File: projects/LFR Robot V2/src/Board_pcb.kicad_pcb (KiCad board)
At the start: 2 copper layers, 77.5 x 103 mm, 0 parts

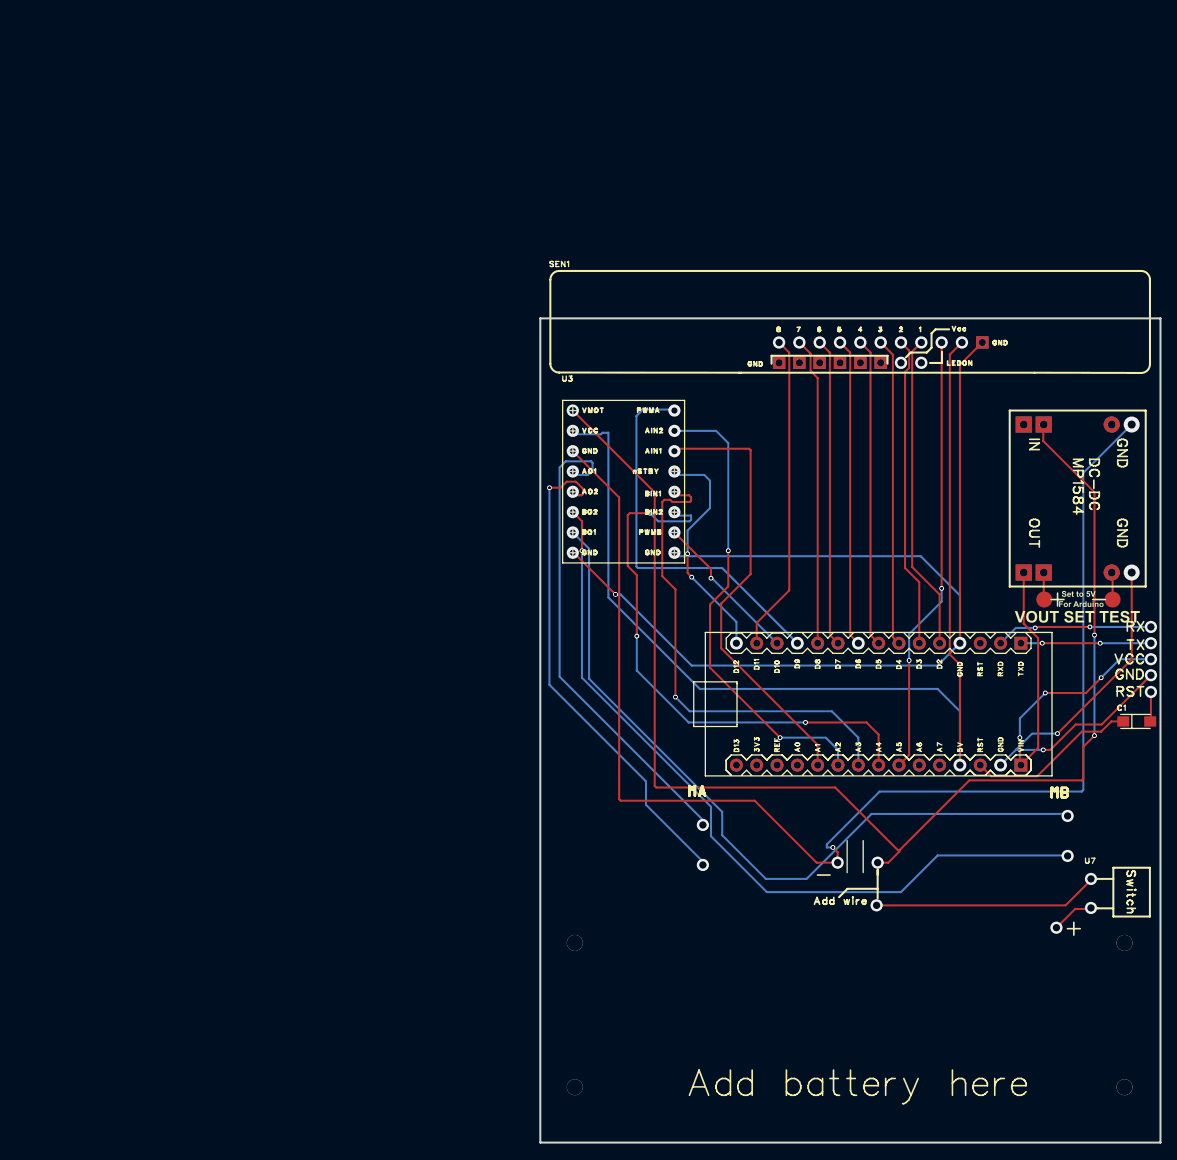
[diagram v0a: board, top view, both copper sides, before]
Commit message: Add files via upload
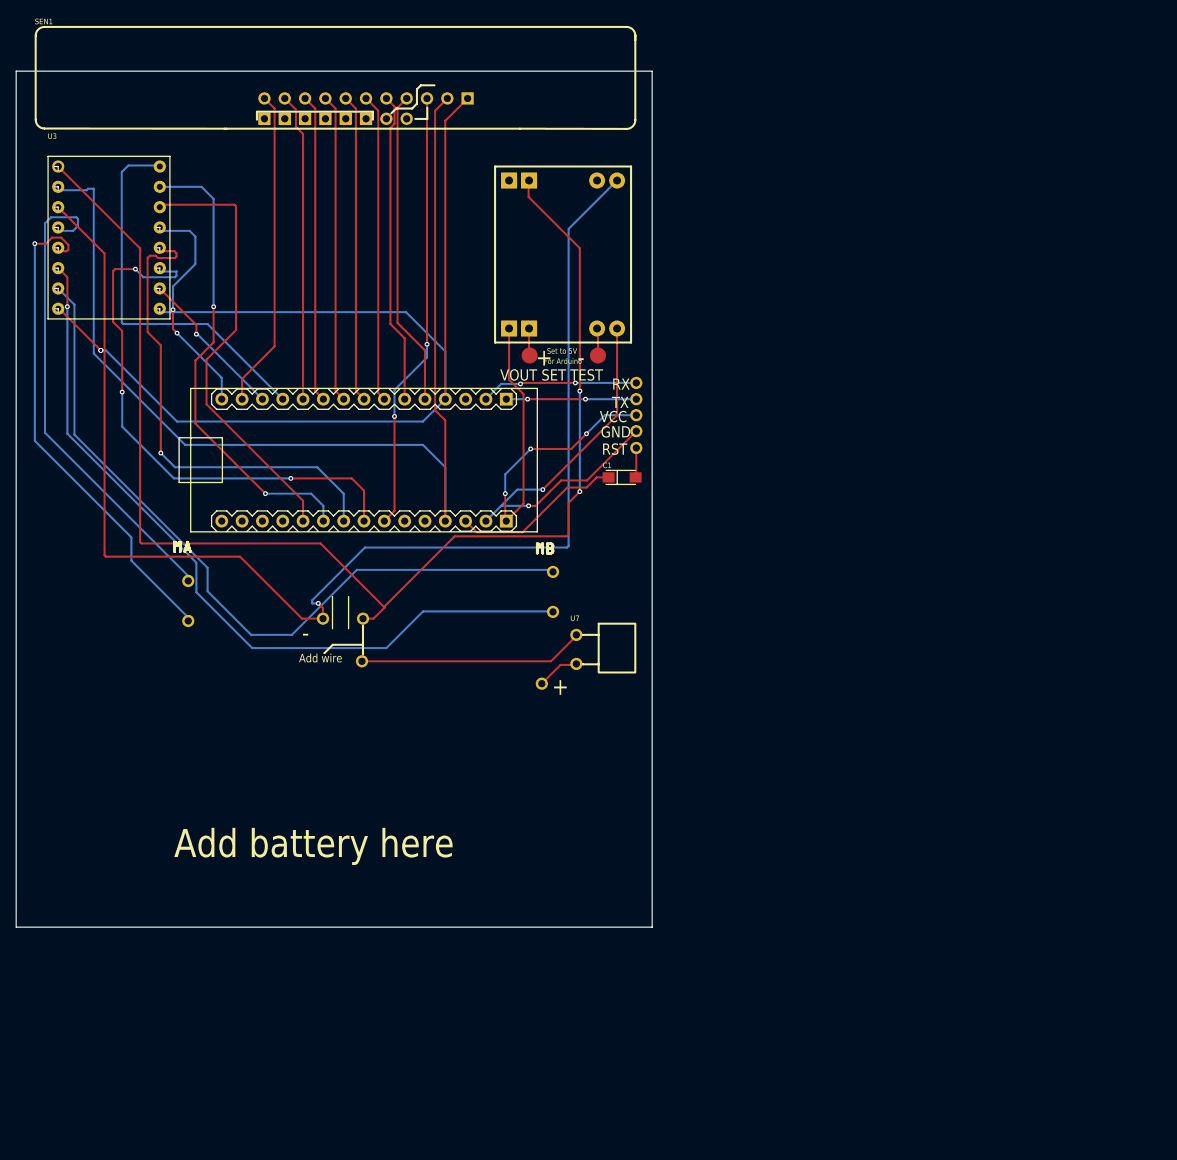
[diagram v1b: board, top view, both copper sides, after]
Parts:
- added ?: , LFR V2:Pad_e140, F.Cu at (195.5, 79.1)
- added ?: , LFR V2:Pad_e431, F.Cu at (195.5, 77.0)
- added ?: , LFR V2:Pad_e429, F.Cu at (195.5, 73.0)
- added ?: , LFR V2:Pad_e428, F.Cu at (195.5, 71.0)
- added ?: , LFR V2:Pad_e194, F.Cu at (183.7, 108.6)
- added ?: , LFR V2:Pad_e430, F.Cu at (195.5, 75.0)
- added ?: , LFR V2:Pad_e33, F.Cu at (161.2, 105.8)
- added ?: , LFR V2:Pad_e235, F.Cu at (190.7, 67.5)
- added ?: , LFR V2:Pad_e234, F.Cu at (182.2, 67.5)
- added C1: , LFR V2:CAP-SMD_L3.2-W1.6-RD, F.Cu at (193.7, 82.8)
- added SEN1: , LFR V2:QTR-8X, F.Cu at (121.1, 45.6)
- added U1: , LFR V2:COMM-TH_ARDUINO_NANO, F.Cu at (161.5, 80.6)
- added U2: , LFR V2:MP1584 BREAKOUT, F.Cu at (177.9, 43.9)
- added U3: , LFR V2:TB6612FNG, F.Cu at (121.9, 63.0)
- added U4: , LFR V2:2PIN SCREW TERMINAL, B.Cu at (139.5, 95.7)
- added U5: , LFR V2:2PIN SCREW TERMINAL, B.Cu at (185.1, 94.6)
- added U6: , LFR V2:2PIN SCREW TERMINAL, B.Cu at (161.4, 100.4)
- added U7: , LFR V2:SwitchOnOff, F.Cu at (193.1, 104.2)
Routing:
- net (no net): track 0.00 -> 1816.5 mm, vias 168 -> 38
- net 0: track 1816.5 -> 0.00 mm
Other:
- board size 77.5 x 103 mm -> 79.5 x 107 mm
- board text added: "+"
- board text added: "-"
- board text added: "03371240723"
- board text added: "Add battery here"
- board text added: "Add wire"
- board text added: "For Arduino"
- board text added: "GND"
- board text added: "RST"
- board text added: "RX"
- board text added: "Set to 5V"
- board text added: "TX"
- board text added: "VCC"
- board text added: "VOUT SET TEST"
- board text added: "techsbazaar.com"
- board text added: "techsbazaarpk"
